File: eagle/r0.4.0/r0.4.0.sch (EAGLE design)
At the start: 8 parts

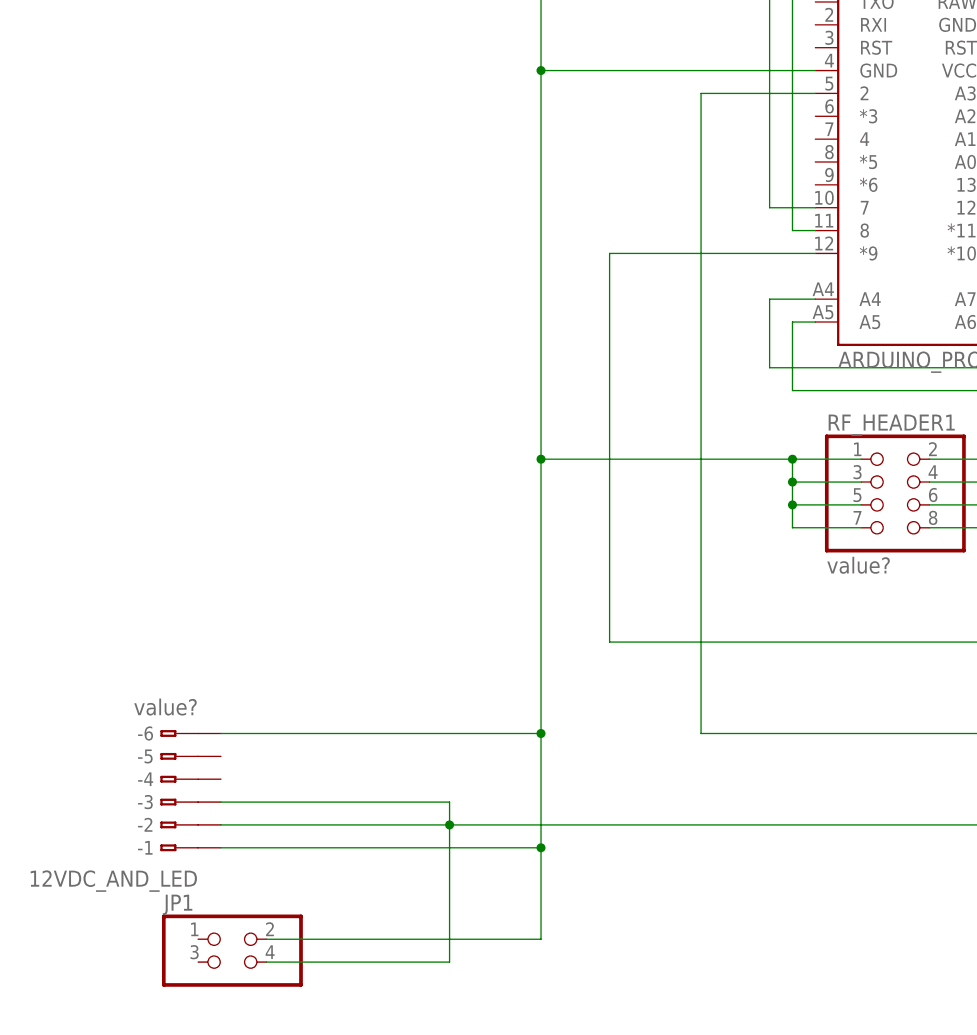
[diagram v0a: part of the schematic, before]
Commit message: Added finishing touches to r0.4.0 of the board
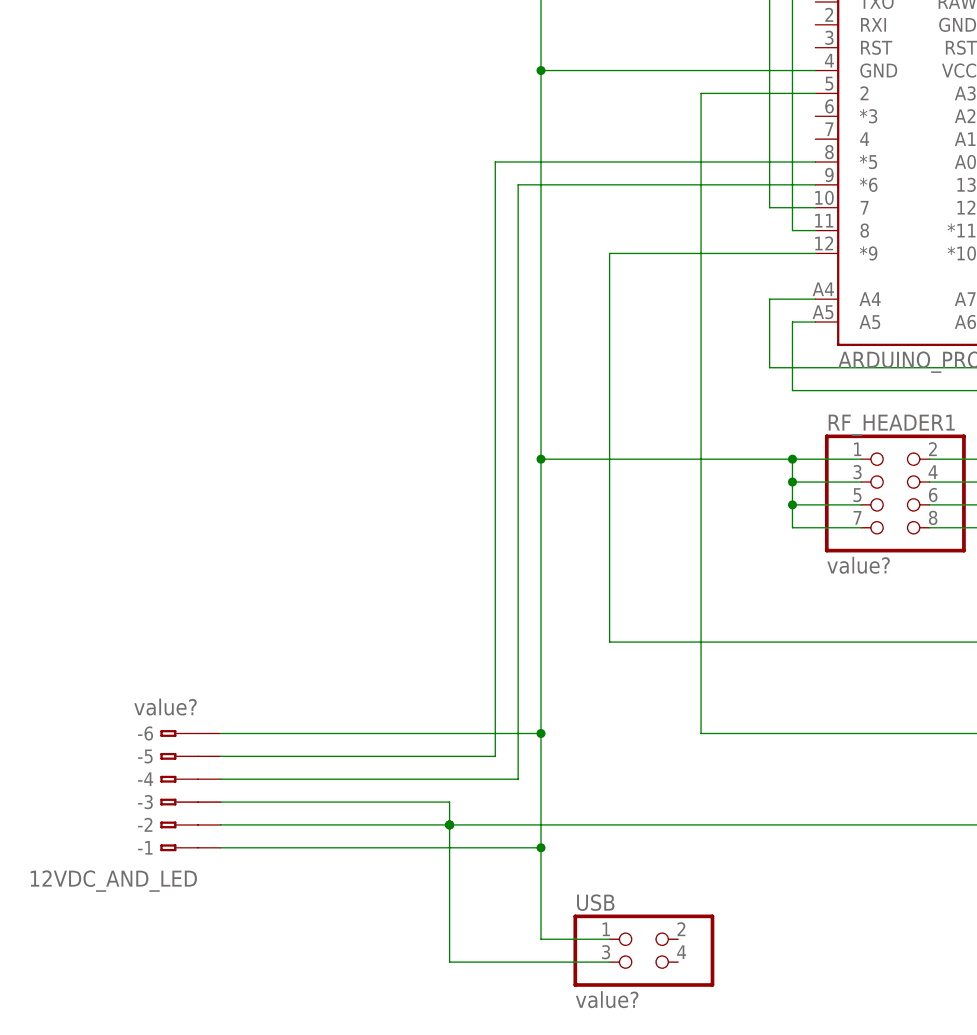
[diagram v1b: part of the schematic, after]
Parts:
- removed JP1: (no value), pinhead:PINHD-2X2
- added USB: value?, pinhead:PINHD-2X2
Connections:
- new net N$4: 12VDC_AND_LED.B-1, 12VDC_AND_LED.B-6, RF_HEADER1.1, RF_HEADER1.3, RF_HEADER1.5, RF_HEADER1.7, U$1.GND, USB.1, X_TILT.2
- new net N$7: 12VDC_AND_LED.B-5, U$1.*5
- net N$11: now also 12VDC_AND_LED.B-4, U$1.*6; no longer 12VDC_AND_LED.B-1, 12VDC_AND_LED.B-6, JP1.2, RF_HEADER1.1, RF_HEADER1.3, RF_HEADER1.5, RF_HEADER1.7, U$1.GND, X_TILT.2
- net N$9: now also USB.3; no longer JP1.4
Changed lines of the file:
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@@
 <part name="RF_HEADER1" library="rf-header" deviceset="PINHD-2X4" device="" value="value?"/>
 <part name="12VDC_AND_LED" library="con-wago" deviceset="234-206" device="" value="value?"/>
-<part name="JP1" library="pinhead" deviceset="PINHD-2X2" device=""/>
+<part name="USB" library="pinhead" deviceset="PINHD-2X2" device="" value="value?"/>
 </parts>
 <sheets>
@@
 <instance part="RF_HEADER1" gate="A" x="5.08" y="17.78"/>
 <instance part="12VDC_AND_LED" gate="G$1" x="-76.2" y="-15.24" rot="R180"/>
-<instance part="JP1" gate="A" x="-66.04" y="-33.02"/>
+<instance part="USB" gate="A" x="-20.32" y="-33.02"/>
 </instances>
 <busses>
@@
 <junction x="-43.18" y="-17.78"/>
 <pinref part="12VDC_AND_LED" gate="G$1" pin="B-2"/>
+<pinref part="12VDC_AND_LED" gate="G$1" pin="B-3"/>
 <wire x1="-43.18" y1="-17.78" x2="-68.58" y2="-17.78" width="0.1524" layer="91"/>
-<pinref part="12VDC_AND_LED" gate="G$1" pin="B-3"/>
 <wire x1="-68.58" y1="-15.24" x2="-43.18" y2="-15.24" width="0.1524" layer="91"/>
-<pinref part="JP1" gate="A" pin="4"/>
-<wire x1="-63.5" y1="-33.02" x2="-43.18" y2="-33.02" width="0.1524" layer="91"/>
-<wire x1="-43.18" y1="-33.02" x2="-43.18" y2="-17.78" width="0.1524" layer="91"/>
+<junction x="-43.18" y="-17.78"/>
+<wire x1="-43.18" y1="-17.78" x2="-43.18" y2="-33.02" width="0.1524" layer="91"/>
+<pinref part="USB" gate="A" pin="3"/>
+<wire x1="-43.18" y1="-33.02" x2="-25.4" y2="-33.02" width="0.1524" layer="91"/>
 </segment>
 </net>
@@
 </segment>
 </net>
-<net name="N$11" class="0">
+<net name="N$12" class="0">
+<segment>
+<pinref part="U$1" gate="G$1" pin="A4"/>
+<wire x1="-2.54" y1="40.64" x2="-7.62" y2="40.64" width="0.1524" layer="91"/>
+<wire x1="-7.62" y1="40.64" x2="-7.62" y2="33.02" width="0.1524" layer="91"/>
+<wire x1="-7.62" y1="33.02" x2="20.32" y2="33.02" width="0.1524" layer="91"/>
+<wire x1="20.32" y1="33.02" x2="20.32" y2="20.32" width="0.1524" layer="91"/>
+<pinref part="RF_HEADER1" gate="A" pin="4"/>
+<wire x1="20.32" y1="20.32" x2="10.16" y2="20.32" width="0.1524" layer="91"/>
+</segment>
+</net>
+<net name="N$18" class="0">
+<segment>
+<pinref part="U$1" gate="G$1" pin="A5"/>
+<wire x1="-2.54" y1="38.1" x2="-5.08" y2="38.1" width="0.1524" layer="91"/>
+<wire x1="-5.08" y1="38.1" x2="-5.08" y2="30.48" width="0.1524" layer="91"/>
+<wire x1="-5.08" y1="30.48" x2="17.78" y2="30.48" width="0.1524" layer="91"/>
+<wire x1="17.78" y1="30.48" x2="17.78" y2="22.86" width="0.1524" layer="91"/>
+<pinref part="RF_HEADER1" gate="A" pin="2"/>
+<wire x1="17.78" y1="22.86" x2="10.16" y2="22.86" width="0.1524" layer="91"/>
+</segment>
+</net>
+<net name="N$19" class="0">
+<segment>
+<pinref part="U$1" gate="G$1" pin="A6"/>
+<wire x1="20.32" y1="38.1" x2="22.86" y2="38.1" width="0.1524" layer="91"/>
+<wire x1="22.86" y1="38.1" x2="22.86" y2="15.24" width="0.1524" layer="91"/>
+<pinref part="RF_HEADER1" gate="A" pin="8"/>
+<wire x1="22.86" y1="15.24" x2="10.16" y2="15.24" width="0.1524" layer="91"/>
+</segment>
+</net>
+<net name="N$20" class="0">
+<segment>
+<pinref part="U$1" gate="G$1" pin="A7"/>
+<wire x1="20.32" y1="40.64" x2="25.4" y2="40.64" width="0.1524" layer="91"/>
+<wire x1="25.4" y1="40.64" x2="25.4" y2="17.78" width="0.1524" layer="91"/>
+<pinref part="RF_HEADER1" gate="A" pin="6"/>
+<wire x1="25.4" y1="17.78" x2="10.16" y2="17.78" width="0.1524" layer="91"/>
+</segment>
+</net>
+<net name="N$4" class="0">
 <segment>
 <pinref part="RF_HEADER1" gate="A" pin="1"/>
@@
 <wire x1="-33.02" y1="22.86" x2="-33.02" y2="-7.62" width="0.1524" layer="91"/>
 <wire x1="-33.02" y1="-7.62" x2="-33.02" y2="-20.32" width="0.1524" layer="91"/>
-<wire x1="-33.02" y1="-20.32" x2="-33.02" y2="-30.48" width="0.1524" layer="91"/>
 <pinref part="U$1" gate="G$1" pin="GND"/>
 <wire x1="-33.02" y1="66.04" x2="-2.54" y2="66.04" width="0.1524" layer="91"/>
@@
 <pinref part="12VDC_AND_LED" gate="G$1" pin="B-1"/>
 <wire x1="-68.58" y1="-20.32" x2="-33.02" y2="-20.32" width="0.1524" layer="91"/>
-<junction x="-33.02" y="-20.32"/>
-<pinref part="JP1" gate="A" pin="2"/>
-<wire x1="-63.5" y1="-30.48" x2="-33.02" y2="-30.48" width="0.1524" layer="91"/>
 <pinref part="12VDC_AND_LED" gate="G$1" pin="B-6"/>
 <wire x1="-68.58" y1="-7.62" x2="-33.02" y2="-7.62" width="0.1524" layer="91"/>
 <junction x="-33.02" y="-7.62"/>
-</segment>
-</net>
-<net name="N$12" class="0">
-<segment>
-<pinref part="U$1" gate="G$1" pin="A4"/>
-<wire x1="-2.54" y1="40.64" x2="-7.62" y2="40.64" width="0.1524" layer="91"/>
-<wire x1="-7.62" y1="40.64" x2="-7.62" y2="33.02" width="0.1524" layer="91"/>
-<wire x1="-7.62" y1="33.02" x2="20.32" y2="33.02" width="0.1524" layer="91"/>
-<wire x1="20.32" y1="33.02" x2="20.32" y2="20.32" width="0.1524" layer="91"/>
-<pinref part="RF_HEADER1" gate="A" pin="4"/>
-<wire x1="20.32" y1="20.32" x2="10.16" y2="20.32" width="0.1524" layer="91"/>
-</segment>
-</net>
-<net name="N$18" class="0">
-<segment>
-<pinref part="U$1" gate="G$1" pin="A5"/>
-<wire x1="-2.54" y1="38.1" x2="-5.08" y2="38.1" width="0.1524" layer="91"/>
-<wire x1="-5.08" y1="38.1" x2="-5.08" y2="30.48" width="0.1524" layer="91"/>
-<wire x1="-5.08" y1="30.48" x2="17.78" y2="30.48" width="0.1524" layer="91"/>
-<wire x1="17.78" y1="30.48" x2="17.78" y2="22.86" width="0.1524" layer="91"/>
-<pinref part="RF_HEADER1" gate="A" pin="2"/>
-<wire x1="17.78" y1="22.86" x2="10.16" y2="22.86" width="0.1524" layer="91"/>
-</segment>
-</net>
-<net name="N$19" class="0">
-<segment>
-<pinref part="U$1" gate="G$1" pin="A6"/>
-<wire x1="20.32" y1="38.1" x2="22.86" y2="38.1" width="0.1524" layer="91"/>
-<wire x1="22.86" y1="38.1" x2="22.86" y2="15.24" width="0.1524" layer="91"/>
-<pinref part="RF_HEADER1" gate="A" pin="8"/>
-<wire x1="22.86" y1="15.24" x2="10.16" y2="15.24" width="0.1524" layer="91"/>
-</segment>
-</net>
-<net name="N$20" class="0">
-<segment>
-<pinref part="U$1" gate="G$1" pin="A7"/>
-<wire x1="20.32" y1="40.64" x2="25.4" y2="40.64" width="0.1524" layer="91"/>
-<wire x1="25.4" y1="40.64" x2="25.4" y2="17.78" width="0.1524" layer="91"/>
-<pinref part="RF_HEADER1" gate="A" pin="6"/>
-<wire x1="25.4" y1="17.78" x2="10.16" y2="17.78" width="0.1524" layer="91"/>
-</segment>
-</net>
+<pinref part="USB" gate="A" pin="1"/>
+<wire x1="-25.4" y1="-30.48" x2="-33.02" y2="-30.48" width="0.1524" layer="91"/>
+<wire x1="-33.02" y1="-30.48" x2="-33.02" y2="-20.32" width="0.1524" layer="91"/>
+<junction x="-33.02" y="-20.32"/>
+</segment>
+</net>
+<net name="N$7" class="0">
+<segment>
+<pinref part="U$1" gate="G$1" pin="*5"/>
+<wire x1="-2.54" y1="55.88" x2="-38.1" y2="55.88" width="0.1524" layer="91"/>
+<wire x1="-38.1" y1="55.88" x2="-38.1" y2="-10.16" width="0.1524" layer="91"/>
+<pinref part="12VDC_AND_LED" gate="G$1" pin="B-5"/>
+<wire x1="-38.1" y1="-10.16" x2="-68.58" y2="-10.16" width="0.1524" layer="91"/>
+</segment>
+</net>
+<net name="N$11" class="0">
+<segment>
+<pinref part="12VDC_AND_LED" gate="G$1" pin="B-4"/>
+<wire x1="-35.56" y1="-12.7" x2="-68.58" y2="-12.7" width="0.1524" layer="91"/>
+<pinref part="U$1" gate="G$1" pin="*6"/>
+<wire x1="-2.54" y1="53.34" x2="-35.56" y2="53.34" width="0.1524" layer="91"/>
+<wire x1="-35.56" y1="-12.7" x2="-35.56" y2="53.34" width="0.1524" layer="91"/>
+</segment>
+</net>
